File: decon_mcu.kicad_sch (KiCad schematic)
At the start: 21 parts, among them J1 Conn_01x16, J2 Conn_01x16, J23 Conn_01x02, J3 Conn_01x16, J4 Conn_01x16, J5 Conn_01x18, U1 URB2405YMD-10WR3, U3 STM32F401R_B-C_Tx, U4 AZ1117-3.3

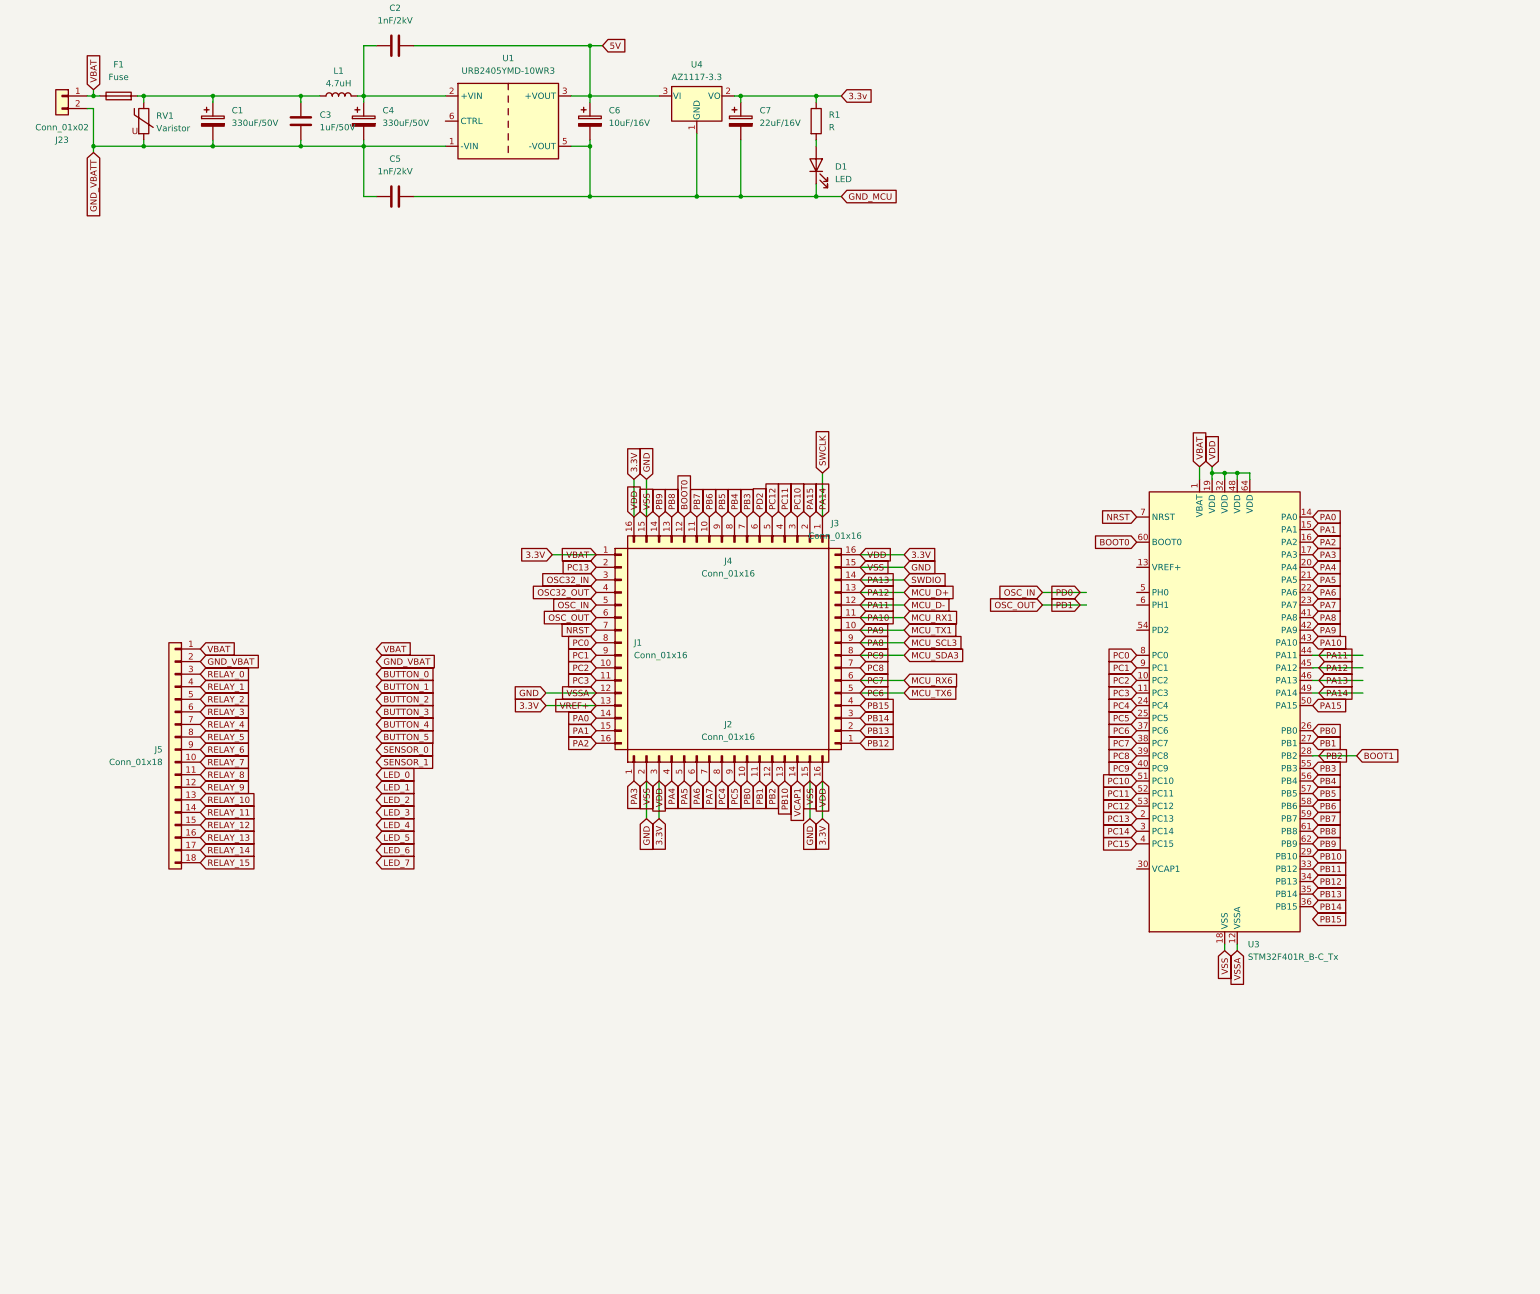
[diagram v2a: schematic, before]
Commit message: modified:   DECON_Ctrl_Panel.kicad_pcb
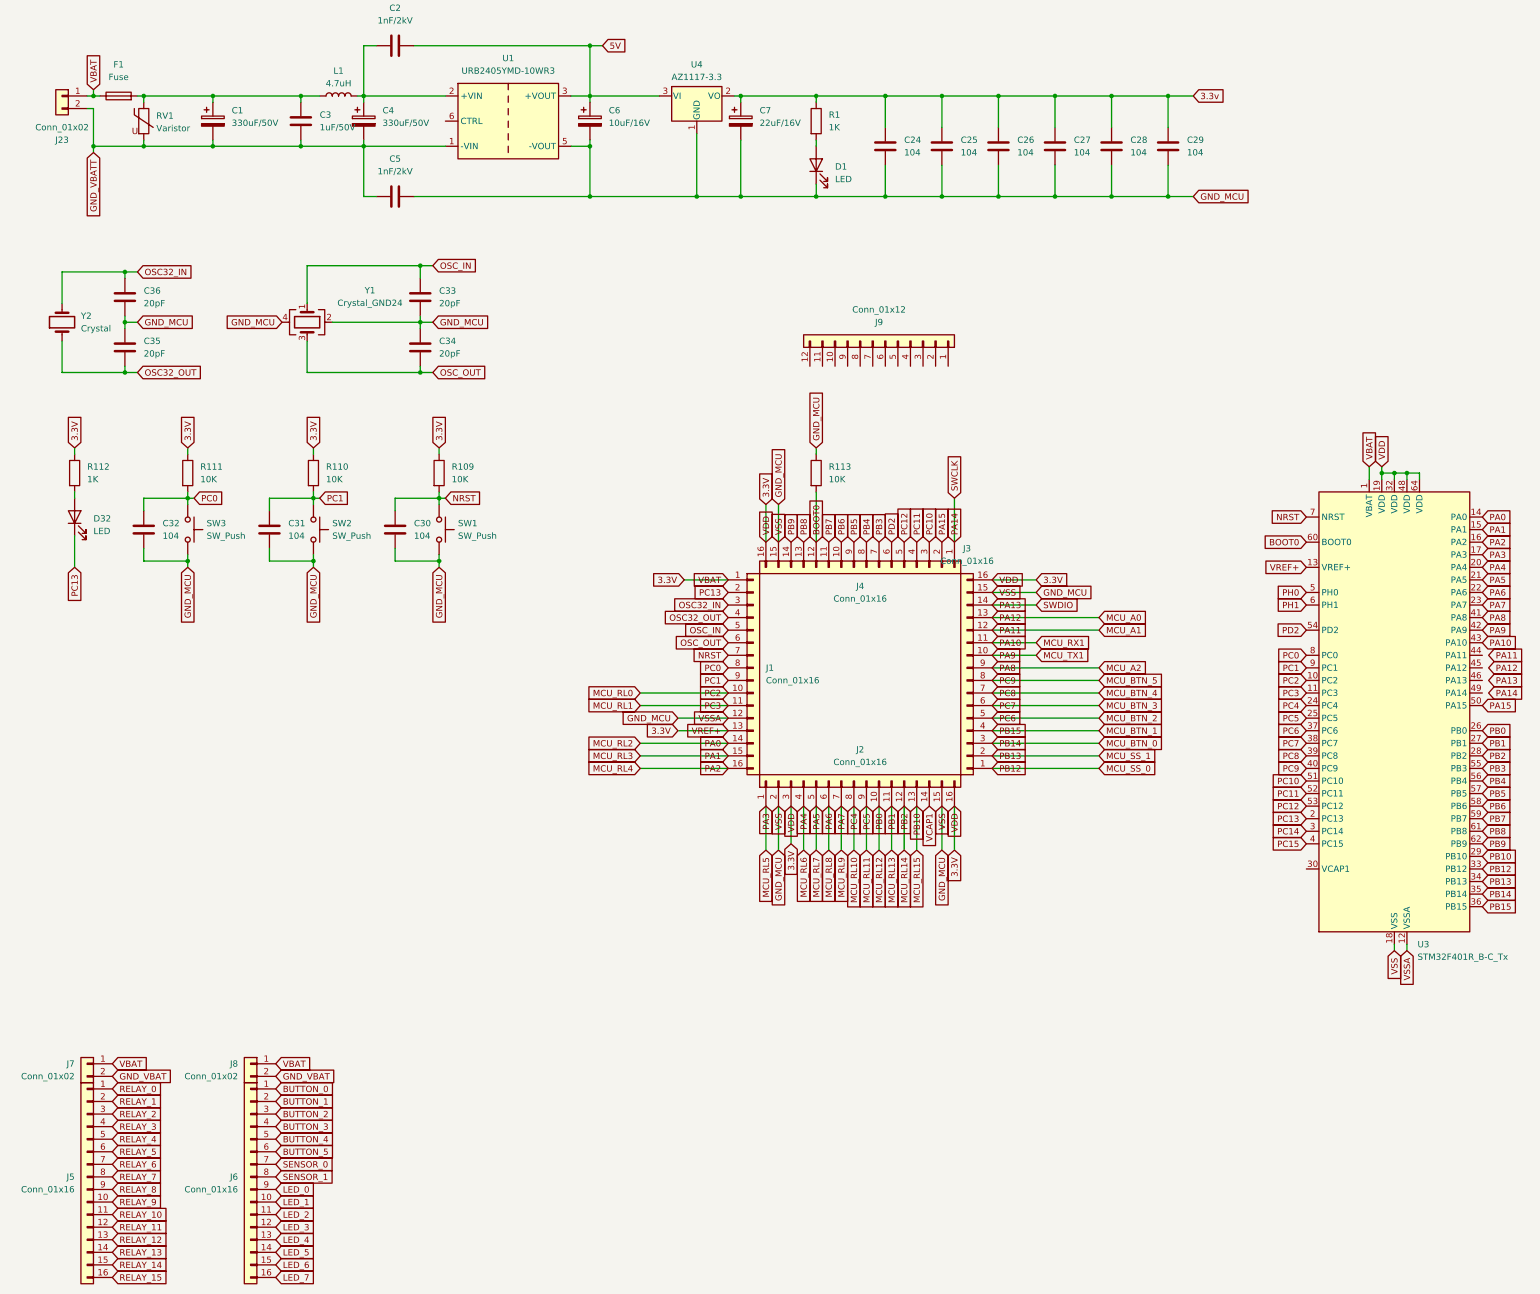
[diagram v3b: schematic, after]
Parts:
- removed J5: Conn_01x18, symbol Connector_Generic:Conn_01x18
- added C24, C25, C26, C27, C28, C29, C30, C31, C32: 104, Capacitor_SMD:C_0805_2012Metric, symbol Device:C
- added C33, C34, C35, C36: 20pF, Capacitor_SMD:C_0805_2012Metric, symbol Device:C
- added D32: LED, LED_SMD:LED_0805_2012Metric, symbol Device:LED
- added J5, J6: Conn_01x16, symbol Connector_Generic:Conn_01x16
- added J7, J8: Conn_01x02, TerminalBlock_Phoenix:TerminalBlock_Phoenix_MKDS-1,5-2-5.08_1x02_P5.08mm_Horizontal, symbol Connector_Generic:Conn_01x02
- added J9: Conn_01x12, Connector_PinHeader_2.54mm:PinHeader_1x12_P2.54mm_Vertical, symbol Connector_Generic:Conn_01x12
- added R109, R110, R111, R113: 10K, symbol Device:R
- added R112: 1K, Resistor_SMD:R_0805_2012Metric, symbol Device:R
- added SW1, SW2, SW3: SW_Push, Button_Switch_SMD:SW_SPST_CK_RS282G05A3, symbol Switch:SW_Push
- added Y1: Crystal_GND24, Crystal:Crystal_SMD_3225-4Pin_3.2x2.5mm, symbol Device:Crystal_GND24
- added Y2: Crystal, Crystal:Crystal_SMD_3215-2Pin_3.2x1.5mm, symbol Device:Crystal
- R1: value R -> 1K
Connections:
- net GND is gone; now on net GND_MCU: J1.12 (Pin_12), J2.15 (Pin_15), J2.2 (Pin_2), J3.15 (Pin_15), J4.15 (Pin_15), U3.12 (VSSA), U3.18 (VSS), U3.31 (VSS), U3.47 (VSS), U3.63 (VSS)
- net PB15 is gone; now on net MCU_BTN_1: J3.4 (Pin_4)
- net 3.3V: now also U3.13 (VREF+), J7.1 (Pin_1), J8.1 (Pin_1), R109.1, R110.1, R111.1, R112.1
- net 3.3v: now also C24.2, C25.2, C26.2, C27.2, C28.2, C29.2
- net BOOT0: now also R113.2
- net BUTTON_0: now also J6.1 (Pin_1)
- net BUTTON_1: now also J6.2 (Pin_2)
- net BUTTON_2: now also J6.3 (Pin_3)
- net BUTTON_3: now also J6.4 (Pin_4)
- net BUTTON_4: now also J6.5 (Pin_5)
- net BUTTON_5: now also J6.6 (Pin_6)
- net GND_MCU: now also C24.1, C25.1, C26.1, C27.1, C28.1, C29.1, C30.2, C31.2, C32.2, C33.1, C34.1, C35.1, C36.2, R113.1, SW1.2, SW2.2, SW3.2, Y1.2, Y1.4
- net GND_VBAT: now also J7.2 (Pin_2), J8.2 (Pin_2)
- net LED_0: now also J6.9 (Pin_9)
- net LED_1: now also J6.10 (Pin_10)
- net LED_2: now also J6.11 (Pin_11)
- net LED_3: now also J6.12 (Pin_12)
- net LED_4: now also J6.13 (Pin_13)
- net LED_5: now also J6.14 (Pin_14)
- net LED_6: now also J6.15 (Pin_15)
- net LED_7: now also J6.16 (Pin_16)
- net NRST: now also C30.1, R109.2, SW1.1
- net OSC32_IN: now also C36.1, Y2.2
- net OSC32_OUT: now also C35.2, Y2.1
- net OSC_IN: now also C33.2, Y1.1
- net OSC_OUT: now also C34.2, Y1.3
- net PA13: no longer U3.46 (PA13)
- net PA14: no longer U3.49 (PA14)
- net PC0: now also C32.1, R111.2, SW3.1
- net PC1: now also C31.1, R110.2, SW2.1
- net PC13: now also D32.1 (K)
- net PD2: now also U3.54 (PD2)
- net RELAY_0: now also J5.1 (Pin_1)
- net RELAY_1: now also J5.2 (Pin_2)
- net RELAY_10: now also J5.11 (Pin_11)
- net RELAY_11: now also J5.12 (Pin_12)
- net RELAY_12: now also J5.13 (Pin_13)
- net RELAY_13: now also J5.14 (Pin_14)
- net RELAY_14: now also J5.15 (Pin_15)
- net RELAY_15: now also J5.16 (Pin_16)
- net RELAY_2: now also J5.3 (Pin_3)
- net RELAY_3: now also J5.4 (Pin_4)
- net RELAY_4: now also J5.5 (Pin_5)
- net RELAY_5: now also J5.6 (Pin_6)
- net RELAY_6: now also J5.7 (Pin_7)
- net RELAY_7: now also J5.8 (Pin_8)
- net RELAY_8: now also J5.9 (Pin_9)
- net RELAY_9: now also J5.10 (Pin_10)
- net SENSOR_0: now also J6.7 (Pin_7)
- net SENSOR_1: now also J6.8 (Pin_8)
- net PH0: now reaches U3.5 (PH0)
- net PH1: now reaches U3.6 (PH1)
- net BOOT1 renamed MCU_RL14
- net MCU_D+: no longer names the net of U3.45 (PA12)
- net MCU_D+: no longer J3.13 (Pin_13)
- net MCU_D-: no longer names the net of U3.44 (PA11)
- net MCU_D-: no longer J3.12 (Pin_12)
- net MCU_RX6 renamed MCU_BTN_3
- net MCU_SCL3 renamed MCU_A2
- net MCU_SDA3 renamed MCU_BTN_5
- net MCU_TX6 renamed MCU_BTN_2
- net PA0 renamed MCU_RL2
- net PA1 renamed MCU_RL3
- net PA2 renamed MCU_RL4
- net PA3 renamed MCU_RL5
- net PA4 renamed MCU_RL6
- net PA5 renamed MCU_RL7
- net PA6 renamed MCU_RL8
- net PA7 renamed MCU_RL9
- net PB0 renamed MCU_RL12
- net PB1 renamed MCU_RL13
- net PB10 renamed MCU_RL15
- net PB11 renamed MCU_SS_0
- net MCU_SS_0: now also J3.1 (Pin_1)
- net PB12 renamed MCU_SS_1
- net MCU_SS_1: now also J3.2 (Pin_2); no longer J3.1 (Pin_1)
- net PB13 renamed MCU_BTN_0
- net MCU_BTN_0: now also J3.3 (Pin_3); no longer J3.2 (Pin_2)
- net PB14 renamed MCU_BTN_1
- net MCU_BTN_1: no longer J3.3 (Pin_3)
- net PC2 renamed MCU_RL0
- net PC3 renamed MCU_RL1
- net PC4 renamed MCU_RL10
- net PC5 renamed MCU_RL11
- net PC8 renamed MCU_BTN_4
- new net: D32.2 (A), R112.2
- new net MCU_A0: J3.13 (Pin_13)
- new net MCU_A1: J3.12 (Pin_12)
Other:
- moved on the sheet: J1, J2, J3, J4, U3

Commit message: modified:   DECON_Ctrl_Panel.kicad_pcb
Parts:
- removed C32: 104, Capacitor_SMD:C_0805_2012Metric, symbol Device:C
- removed J23: Conn_01x02, symbol Connector_Generic:Conn_01x02
- removed J5, J6: Conn_01x16, symbol Connector_Generic:Conn_01x16
- removed J7, J8: Conn_01x02, TerminalBlock_Phoenix:TerminalBlock_Phoenix_MKDS-1,5-2-5.08_1x02_P5.08mm_Horizontal, symbol Connector_Generic:Conn_01x02
- removed R111: 10K, symbol Device:R
- removed SW3: SW_Push, Button_Switch_SMD:SW_SPST_CK_RS282G05A3, symbol Switch:SW_Push
- added C13: 104, Capacitor_SMD:C_0805_2012Metric, symbol Device:C
- added C21: 2.2uF, Capacitor_SMD:C_0805_2012Metric, symbol Device:C
- added J10, J18, J19, J9: Conn_01x03, symbol Connector_Generic:Conn_01x03
- added J11, J12, J14, J15, J16, J7, J8: Conn_01x06, TerminalBlock_MetzConnect:TerminalBlock_MetzConnect_Type086_RT03406HBLC_1x06_P3.81mm_Horizontal, symbol Connector_Generic:Conn_01x06
- added J13: Conn_01x02, TerminalBlock_MetzConnect:TerminalBlock_MetzConnect_Type086_RT03402HBLC_1x02_P3.81mm_Horizontal, symbol Connector_Generic:Conn_01x02
- added J17: Conn_01x04, symbol Connector_Generic:Conn_01x04
- added J5: FLASH, Connector_PinHeader_1.00mm:PinHeader_1x08_P1.00mm_Vertical, symbol Connector_Generic:Conn_01x08
- J4: renamed from J9; value Conn_01x12 -> GPIO
- R2: renamed from R113; footprint (none) -> Resistor_SMD:R_0805_2012Metric
- R4: renamed from R110; footprint (none) -> Resistor_SMD:R_0805_2012Metric
- R5: renamed from R109; footprint (none) -> Resistor_SMD:R_0805_2012Metric
- renumbered C2 to C1, C27 to C10, C28 to C11, C29 to C12, C5 to C14, C36 to C15, C33 to C16, C31 to C17, C30 to C18, C35 to C19, C1 to C2, C34 to C20, C6 to C5, C7 to C6, C24 to C7, C25 to C8, C26 to C9, D32 to D2, J4 to J1, J1 to J2, J2 to J6, R112 to R3, SW2 to SW1, SW1 to SW2, U4 to U1, U1 to U2, Y2 to Y1, Y1 to Y2
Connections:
- net 3.3v is gone; now on net 3.3V: C10.2, C11.2, C12.2, C6.1, C7.2, C8.2, C9.2, R1.1, U1.2 (VO)
- net MCU_BTN_5 is gone; now on net MCU_A0: J3.8 (Pin_8), U3.40 (PC9)
- net PC0 is gone; now on net MCU_RL0: J2.8 (Pin_8), U3.8 (PC0)
- net 3.3V: now also C13.2, J5.5 (Pin_5); no longer F1.1
- net BUTTON_0: now also J11.1 (Pin_1), J7.4 (Pin_4)
- net BUTTON_1: now also J11.2 (Pin_2), J7.5 (Pin_5)
- net BUTTON_2: now also J11.3 (Pin_3), J7.6 (Pin_6)
- net BUTTON_3: now also J11.4 (Pin_4), J8.1 (Pin_1)
- net GND_MCU: now also C13.1, C21.2, J5.1 (Pin_1), J5.8 (Pin_8)
- net GND_VBAT: now also J10.2 (Pin_2), J13.2 (Pin_2), J14.1 (Pin_1), J16.6 (Pin_6), J17.4 (Pin_4), J18.3 (Pin_3), J19.2 (Pin_2), J7.2 (Pin_2)
- net LED_0: now also J11.6 (Pin_6), J8.3 (Pin_3)
- net LED_1: now also J12.1 (Pin_1), J8.4 (Pin_4)
- net LED_2: now also J12.2 (Pin_2), J8.5 (Pin_5)
- net LED_3: now also J12.3 (Pin_3), J8.6 (Pin_6)
- net LED_4: now also J12.4 (Pin_4), J9.1 (Pin_1)
- net LED_5: now also J12.5 (Pin_5), J9.2 (Pin_2)
- net LED_6: now also J12.6 (Pin_6), J9.3 (Pin_3)
- net MCU_A0: no longer J3.13 (Pin_13)
- net MCU_A1: now also J3.7 (Pin_7), U3.39 (PC8); no longer J3.12 (Pin_12)
- net MCU_A2: now also J3.6 (Pin_6), U3.38 (PC7); no longer J3.9 (Pin_9), U3.41 (PA8)
- net MCU_BTN_0: now also J3.1 (Pin_1), U3.33 (PB12); no longer J3.3 (Pin_3), U3.35 (PB14)
- net MCU_BTN_1: now also J3.2 (Pin_2), U3.34 (PB13); no longer J3.4 (Pin_4), U3.36 (PB15)
- net MCU_BTN_2: now also J3.3 (Pin_3), U3.35 (PB14); no longer J3.5 (Pin_5), U3.37 (PC6)
- net MCU_BTN_3: now also J3.4 (Pin_4), U3.36 (PB15); no longer J3.6 (Pin_6), U3.38 (PC7)
- net MCU_BTN_4: now also J3.5 (Pin_5), U3.37 (PC6); no longer J3.7 (Pin_7), U3.39 (PC8)
- net MCU_RL0: no longer J2.10 (Pin_10), U3.10 (PC2)
- net MCU_RL1: now also J2.9 (Pin_9), U3.9 (PC1); no longer J2.11 (Pin_11), U3.11 (PC3)
- net MCU_RL10: now also J6.6 (Pin_6), U3.22 (PA6); no longer J6.8 (Pin_8), U3.24 (PC4)
- net MCU_RL11: now also J6.7 (Pin_7), U3.23 (PA7); no longer J6.9 (Pin_9), U3.25 (PC5)
- net MCU_RL12: now also J6.8 (Pin_8), U3.24 (PC4); no longer J6.10 (Pin_10), U3.26 (PB0)
- net MCU_RL13: now also J6.9 (Pin_9), U3.25 (PC5); no longer J6.11 (Pin_11), U3.27 (PB1)
- net MCU_RL14: now also J6.10 (Pin_10), U3.26 (PB0); no longer J6.12 (Pin_12), U3.28 (PB2)
- net MCU_RL15: now also J6.11 (Pin_11), U3.27 (PB1); no longer J6.13 (Pin_13), U3.29 (PB10)
- net MCU_RL2: now also J2.10 (Pin_10), U3.10 (PC2); no longer J2.14 (Pin_14), U3.14 (PA0)
- net MCU_RL3: now also J2.11 (Pin_11), U3.11 (PC3); no longer J2.15 (Pin_15), U3.15 (PA1)
- net MCU_RL4: now also J2.14 (Pin_14), U3.14 (PA0); no longer J2.16 (Pin_16), U3.16 (PA2)
- net MCU_RL5: now also J2.15 (Pin_15), U3.15 (PA1); no longer J6.1 (Pin_1), U3.17 (PA3)
- net MCU_RL6: now also J2.16 (Pin_16), U3.16 (PA2); no longer J6.4 (Pin_4), U3.20 (PA4)
- net MCU_RL7: now also J6.1 (Pin_1), U3.17 (PA3); no longer J6.5 (Pin_5), U3.21 (PA5)
- net MCU_RL8: now also J6.4 (Pin_4), U3.20 (PA4); no longer J6.6 (Pin_6), U3.22 (PA6)
- net MCU_RL9: now also J6.5 (Pin_5), U3.21 (PA5); no longer J6.7 (Pin_7), U3.23 (PA7)
- net MCU_RX1: now also J5.7 (Pin_7)
- net MCU_SS_0: now also J6.12 (Pin_12), U3.28 (PB2); no longer J3.1 (Pin_1), U3.33 (PB12)
- net MCU_SS_1: now also J6.13 (Pin_13), U3.29 (PB10); no longer J3.2 (Pin_2), U3.34 (PB13)
- net MCU_TX1: now also J5.6 (Pin_6)
- net NRST: now also J5.2 (Pin_2)
- net PA13: now also J5.4 (Pin_4)
- net PA14: now also J5.3 (Pin_3)
- net PA15: now also J4.1 (Pin_1)
- net PB3: now also J4.6 (Pin_6)
- net PB4: now also J4.7 (Pin_7)
- net PB5: now also J4.8 (Pin_8)
- net PB6: now also J4.9 (Pin_9)
- net PB7: now also J4.10 (Pin_10)
- net PB8: now also J4.11 (Pin_11)
- net PB9: now also J4.12 (Pin_12)
- net PC10: now also J4.2 (Pin_2)
- net PC11: now also J4.3 (Pin_3)
- net PC12: now also J4.4 (Pin_4)
- net PD2: now also J4.5 (Pin_5)
- net RELAY_0: now also J14.2 (Pin_2)
- net RELAY_1: now also J14.3 (Pin_3)
- net RELAY_10: now also J15.6 (Pin_6)
- net RELAY_11: now also J16.1 (Pin_1)
- net RELAY_12: now also J16.2 (Pin_2)
- net RELAY_13: now also J16.3 (Pin_3)
- net RELAY_14: now also J16.4 (Pin_4)
- net RELAY_15: now also J16.5 (Pin_5)
- net RELAY_2: now also J14.4 (Pin_4)
- net RELAY_3: now also J14.5 (Pin_5)
- net RELAY_4: now also J14.6 (Pin_6)
- net RELAY_5: now also J15.1 (Pin_1)
- net RELAY_6: now also J15.2 (Pin_2)
- net RELAY_7: now also J15.3 (Pin_3)
- net RELAY_8: now also J15.4 (Pin_4)
- net RELAY_9: now also J15.5 (Pin_5)
- net SENSOR_0: now also J17.2 (Pin_2)
- net SENSOR_1: now also J17.3 (Pin_3)
- net VCAP1: now also C21.1
- net PC1 renamed MCU_EXTI
- net MCU_EXTI: now also J3.9 (Pin_9), U3.41 (PA8); no longer J2.9 (Pin_9), U3.9 (PC1)
- new net BUTTON_EN: J10.3 (Pin_3), J7.3 (Pin_3)
- new net EXT_INPUT: J19.3 (Pin_3)
- new net EXT_OUTPUT: J18.2 (Pin_2)
- new net LED_POWER: J11.5 (Pin_5), J8.2 (Pin_2)
- new net PA11: J3.12 (Pin_12)
- new net PA12: J3.13 (Pin_13)
- new net VBAT: F1.1, J10.1 (Pin_1), J13.1 (Pin_1), J17.1 (Pin_1), J18.1 (Pin_1), J19.1 (Pin_1), J7.1 (Pin_1)
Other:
- note added: "CONNECTOR"
- note added: "MCU"
- note added: "POWER"
- moved on the sheet: C15, C16, C17, C18, C19, C20, D2, J1, J2, J3, J4, J6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
